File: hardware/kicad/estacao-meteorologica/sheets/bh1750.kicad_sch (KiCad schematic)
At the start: 10 parts, among them Q1 NMOS, U9 BH1750FVI-TR

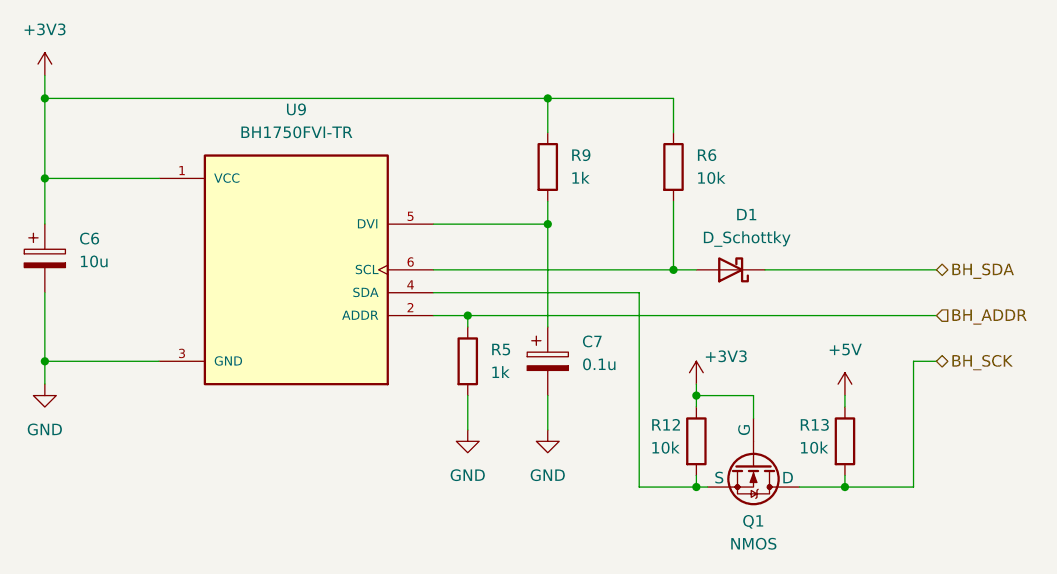
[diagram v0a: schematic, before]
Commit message: refatoracao: atualizacoes de hardware e falta revisao LoRa
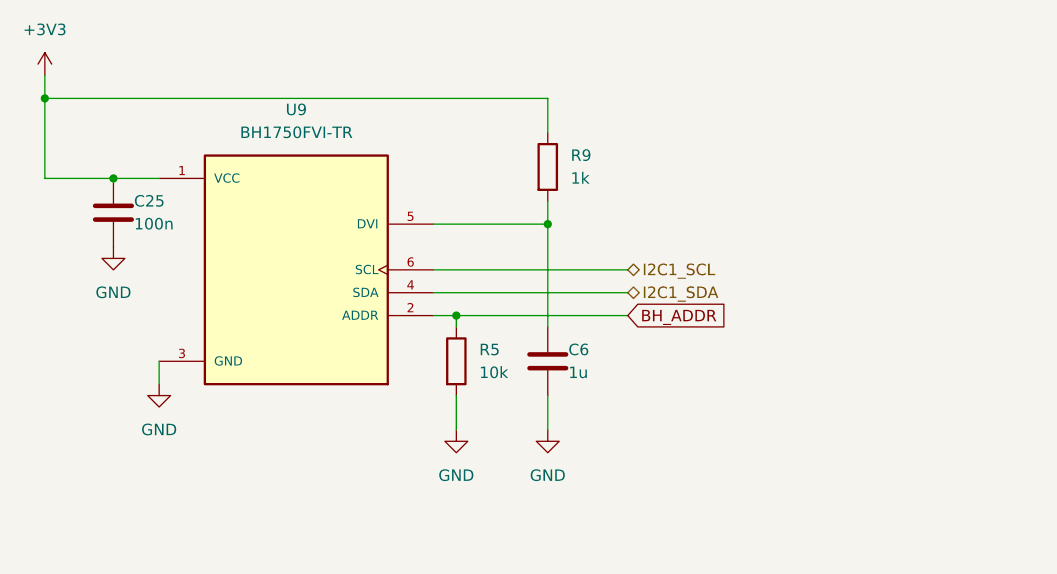
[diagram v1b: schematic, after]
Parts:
- removed C6: 10u, symbol Device:C_Polarized
- removed C7: 0.1u, symbol Device:C_Polarized
- removed D1: D_Schottky, symbol Device:D_Schottky
- removed Q1: NMOS, symbol Simulation_SPICE:NMOS
- removed R12, R13, R6: 10k, symbol Device:R
- added C25: 100n, Capacitor_SMD:C_0603_1608Metric, symbol Device:C
- added C6: 1u, Capacitor_SMD:C_0603_1608Metric, symbol Device:C
- R5: value 1k -> 10k; footprint (none) -> Resistor_SMD:R_0603_1608Metric; Function (none) -> Pull-down opcional de ADDR; hoje está em paralelo ao strap 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; LCSC (none) -> C25804; LCSC Part (none) -> C25804; MPN (none) -> 0603WAF1002T5E; Manufacturer (none) -> UNI-ROYAL; Rating (none) -> 10 kOhm; 1%; 0,1 W; 75 V; 0603
- R9: footprint (none) -> Resistor_SMD:R_0603_1608Metric; Function (none) -> Resistor do RC de partida no pino DVI do BH1750.; LCSC (none) -> C21190; LCSC Part (none) -> C21190; MPN (none) -> 0603WAF1001T5E; Manufacturer (none) -> UNI-ROYAL; Rating (none) -> 1 kOhm; 1%; 0,1 W; 75 V; 0603
- U9: footprint myLibrary:BH1750FVI-TR_sensor -> Hardware_Sensors:BH1750FVI-TR_WSOF-6; Function (none) -> Sensor de iluminância; ADDR em baixo seleciona o endereço I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; LCSC (none) -> C78960; LCSC Part (none) -> C78960; MPN (none) -> BH1750FVI-TR; Manufacturer (none) -> ROHM Semiconductor; Rating (none) -> 2,4 a 3,6 V; -40 a +85 °C; WSOF-6
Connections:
- net +3V3: now also C25.1
- net GND: now also C25.2, C6.2
- net I2C1_SDA: now reaches U9.4 (SDA)
- net at R9.2, U9.5 (DVI): now also C6.1
- net I2C1_SCL: now reaches U9.6 (SCL)
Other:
- moved on the sheet: R5

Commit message: refatoracao: lora + Verificacao projeto inteiro
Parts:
- C25: Modelo 3D (none) -> ${KICAD9_3DMODEL_DIR}/Capacitor_SMD.3dshapes/C_0603_1608Met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; Status_Ficha (none) -> Conferido no catalogo em 2026-09-24; verificar estoque ao c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
- C6: Manufacturer SAMWHA -> Samwha Capacitor; Modelo 3D (none) -> ${KICAD9_3DMODEL_DIR}/Capacitor_SMD.3dshapes/C_0603_1608Met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; Status_Ficha (none) -> Conferido no catalogo em 2026-09-24; verificar estoque ao c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
- R5: Function Pull-down opcional de ADDR; hoje está em paralelo ao strap 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 -> Pull-down de ADDR do BH1750; seleciona endereco I2C 0x23; Manufacturer UNI-ROYAL -> UNI-ROYAL(Uniroyal Elec); Modelo 3D (none) -> ${KICAD9_3DMODEL_DIR}/Resistor_SMD.3dshapes/R_0603_1608Metr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; Status_Ficha (none) -> Conferido no catalogo em 2026-09-24; verificar estoque ao c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
- R9: Manufacturer UNI-ROYAL -> UNI-ROYAL(Uniroyal Elec); Modelo 3D (none) -> ${KICAD9_3DMODEL_DIR}/Resistor_SMD.3dshapes/R_0603_1608Metr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; Status_Ficha (none) -> Conferido no catalogo em 2026-09-24; verificar estoque ao c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
- U9: Manufacturer ROHM Semiconductor -> ROHM Semicon; Modelo 3D (none) -> ${KIPRJMOD}/../../libraries/Hardware_Sensors/Hardware_Senso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; Status_Ficha (none) -> Conferido no catalogo em 2026-09-24; verificar estoque ao c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
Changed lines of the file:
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@@
 			)
 		)
-		(property "Datasheet" "https://fscdn.rohm.com/en/products/databook/datasheet/ic/sensor/light/bh1750fvi-e.pdf"
-			(at 148.59 97.79 0)
-			(effects
-				(font
-					(size 1.27 1.27)
-				)
-				(hide yes)
-			)
-		)
-		(property "Description" "Sensor digital de iluminância ambiente, I2C, 2,4 a 3,6 V, WSOF-6"
-			(at 148.59 97.79 0)
-			(effects
-				(font
-					(size 1.27 1.27)
-				)
-				(hide yes)
-			)
-		)
-		(property "Manufacturer" "ROHM Semiconductor"
+		(property "Datasheet" "https://www.lcsc.com/datasheet/lcsc_datasheet_1811081611_ROHM-Semicon-BH1750FVI-TR_C78960.pdf"
+			(at 148.59 97.79 0)
+			(effects
+				(font
+					(size 1.27 1.27)
+				)
+				(hide yes)
+			)
+		)
+		(property "Description" "-40℃~+85℃ 2.4V~3.6V 65.535klx I2C Light Intensity WSOF-6 Ambient Light Sensors RoHS"
+			(at 148.59 97.79 0)
+			(effects
+				(font
+					(size 1.27 1.27)
+				)
+				(hide yes)
+			)
+		)
+		(property "Manufacturer" "ROHM Semicon"
 			(at 148.59 97.79 0)
 			(effects
@@
 				)
 				(justify bottom)
+				(hide yes)
+			)
+		)
+		(property "Modelo 3D" "${KIPRJMOD}/../../libraries/Hardware_Sensors/Hardware_Sensors.3dshapes/BH1750FVI-TR.step"
+			(at 148.59 97.79 0)
+			(effects
+				(font
+					(size 1.27 1.27)
+				)
+				(hide yes)
+			)
+		)
+		(property "Status_Ficha" "Conferido no catalogo em 2026-09-24; verificar estoque ao comprar"
+			(at 148.59 97.79 0)
+			(effects
+				(font
+					(size 1.27 1.27)
+				)
+				(hide yes)
+			)
+		)
+		(property "CREATOR" ""
+			(at 148.59 97.79 0)
+			(effects
+				(font
+					(size 1.27 1.27)
+				)
+				(hide yes)
+			)
+		)
+		(property "VERIFIER" ""
+			(at 148.59 97.79 0)
+			(effects
+				(font
+					(size 1.27 1.27)
+				)
 				(hide yes)
 			)
@@
 			)
 		)
-		(property "Datasheet" "https://www.lcsc.com/product-detail/C513775.html"
+		(property "Datasheet" "https://wmsc.lcsc.com/wmsc/upload/file/pdf/v2/lcsc/2005192033_Samwha-Capacitor-CS1608X7R105K250NRB_C513775.pdf"
 			(at 176.53 107.95 0)
 			(effects
@@
 			)
 		)
-		(property "Description" "Capacitor cerâmico 1 uF, X7R, 25 V, 0603"
+		(property "Description" "1uF 25V X7R ±10% 0603 Multilayer Ceramic Capacitors MLCC - SMD/SMT RoHS"
 			(at 176.53 107.95 0)
 			(effects
@@
 			)
 		)
-		(property "Manufacturer" "SAMWHA"
+		(property "Manufacturer" "Samwha Capacitor"
 			(at 176.53 107.95 0)
 			(effects
@@
 		)
 		(property "Function" "Capacitor do RC de partida no pino DVI do BH1750."
+			(at 176.53 107.95 0)
+			(effects
+				(font
+					(size 1.27 1.27)
+				)
+				(hide yes)
+			)
+		)
+		(property "Modelo 3D" "${KICAD9_3DMODEL_DIR}/Capacitor_SMD.3dshapes/C_0603_1608Metric.step"
+			(at 176.53 107.95 0)
+			(effects
+				(font
+					(size 1.27 1.27)
+				)
+				(hide yes)
+			)
+		)
+		(property "Status_Ficha" "Conferido no catalogo em 2026-09-24; verificar estoque ao comprar"
+			(at 176.53 107.95 0)
+			(effects
+				(font
+					(size 1.27 1.27)
+				)
+				(hide yes)
+			)
+		)
+		(property "CREATOR" ""
+			(at 176.53 107.95 0)
+			(effects
+				(font
+					(size 1.27 1.27)
+				)
+				(hide yes)
+			)
+		)
+		(property "VERIFIER" ""
 			(at 176.53 107.95 0)
 			(effects
@@
 			)
 		)
-		(property "Datasheet" "https://www.lcsc.com/product-detail/C25804.html"
+		(property "Datasheet" "https://www.lcsc.com/datasheet/lcsc_datasheet_2206010045_UNI-ROYAL-Uniroyal-Elec-0603WAF1002T5E_C25804.pdf"
 			(at 166.37 107.95 0)
 			(effects
@@
 			)
 		)
-		(property "Description" "Resistor de filme espesso, 10 kOhm, 1%, 0,1 W, 0603"
+		(property "Description" "Resistor SMD 10 kohm, 1%, 0,1 W, 0603"
 			(at 166.37 107.95 0)
 			(effects
@@
 			)
 		)
-		(property "Manufacturer" "UNI-ROYAL"
+		(property "Manufacturer" "UNI-ROYAL(Uniroyal Elec)"
 			(at 166.37 107.95 0)
 			(effects
@@
 			)
 		)
-		(property "Function" "Pull-down opcional de ADDR; hoje está em paralelo ao strap direto para GND da folha raiz (endereço 0x23)."
+		(property "Function" "Pull-down de ADDR do BH1750; seleciona endereco I2C 0x23"
+			(at 166.37 107.95 0)
+			(effects
+				(font
+					(size 1.27 1.27)
+				)
+				(hide yes)
+			)
+		)
+		(property "Modelo 3D" "${KICAD9_3DMODEL_DIR}/Resistor_SMD.3dshapes/R_0603_1608Metric.step"
+			(at 166.37 107.95 0)
+			(effects
+				(font
+					(size 1.27 1.27)
+				)
+				(hide yes)
+			)
+		)
+		(property "Status_Ficha" "Conferido no catalogo em 2026-09-24; verificar estoque ao comprar"
+			(at 166.37 107.95 0)
+			(effects
+				(font
+					(size 1.27 1.27)
+				)
+				(hide yes)
+			)
+		)
+		(property "CREATOR" ""
+			(at 166.37 107.95 0)
+			(effects
+				(font
+					(size 1.27 1.27)
+				)
+				(hide yes)
+			)
+		)
+		(property "VERIFIER" ""
 			(at 166.37 107.95 0)
 			(effects
@@
 			)
 		)
-		(property "Datasheet" "https://www.lcsc.com/product-detail/C21190.html"
+		(property "Datasheet" "https://www.lcsc.com/datasheet/lcsc_datasheet_2206010130_UNI-ROYAL-Uniroyal-Elec-0603WAF1001T5E_C21190.pdf"
 			(at 176.53 86.36 0)
 			(effects
@@
 			)
 		)
-		(property "Description" "Resistor de filme espesso, 1 kOhm, 1%, 0,1 W, 0603"
+		(property "Description" "Resistor SMD 1 kohm, 1%, 0,1 W, 0603"
 			(at 176.53 86.36 0)
 			(effects
@@
 			)
 		)
-		(property "Manufacturer" "UNI-ROYAL"
+		(property "Manufacturer" "UNI-ROYAL(Uniroyal Elec)"
 			(at 176.53 86.36 0)
 			(effects
@@
 		)
 		(property "Function" "Resistor do RC de partida no pino DVI do BH1750."
+			(at 176.53 86.36 0)
+			(effects
+				(font
+					(size 1.27 1.27)
+				)
+				(hide yes)
+			)
+		)
+		(property "Modelo 3D" "${KICAD9_3DMODEL_DIR}/Resistor_SMD.3dshapes/R_0603_1608Metric.step"
+			(at 176.53 86.36 0)
+			(effects
+				(font
+					(size 1.27 1.27)
+				)
+				(hide yes)
+			)
+		)
+		(property "Status_Ficha" "Conferido no catalogo em 2026-09-24; verificar estoque ao comprar"
+			(at 176.53 86.36 0)
+			(effects
+				(font
+					(size 1.27 1.27)
+				)
+				(hide yes)
+			)
+		)
+		(property "CREATOR" ""
+			(at 176.53 86.36 0)
+			(effects
+				(font
+					(size 1.27 1.27)
+				)
+				(hide yes)
+			)
+		)
+		(property "VERIFIER" ""
 			(at 176.53 86.36 0)
 			(effects
@@
 			)
 		)
-		(property "Datasheet" "https://www.lcsc.com/product-detail/C14663.html"
+		(property "Datasheet" "https://www.lcsc.com/datasheet/lcsc_datasheet_2211101700_YAGEO-CC0603KRX7R9BB104_C14663.pdf"
 			(at 128.27 91.44 0)
 			(effects
@@
 			)
 		)
-		(property "Description" "Capacitor cerâmico 100 nF, X7R, 50 V, 0603"
+		(property "Description" "Capacitor ceramico 100 nF, 50 V, X7R, 10%, 0603"
 			(at 128.27 91.44 0)
 			(effects
@@
 			(at 128.27 91.44 0)
 			(effects
+				(font
+					(size 1.27 1.27)
+				)
+				(hide yes)
+			)
+		)
+		(property "Modelo 3D" "${KICAD9_3DMODEL_DIR}/Capacitor_SMD.3dshapes/C_0603_1608Metric.step"
+			(at 128.27 91.44 0)
+			(effects
+				(font
+					(size 1.27 1.27)
+				)
+				(hide yes)
+			)
+		)
+		(property "Status_Ficha" "Conferido no catalogo em 2026-09-24; verificar estoque ao comprar"
+			(at 128.27 91.44 0)
+			(effects
+				(font
+					(size 1.27 1.27)
+				)
+				(hide yes)
+			)
+		)
+		(property "CREATOR" ""
+			(at 128.27 91.44 0)
+			(effects
+				(font
+					(size 1.27 1.27)
+				)
+				(hide yes)
+			)
+		)
+		(property "VERIFIER" ""
+			(at 128.27 91.44 0)
+			(effects
